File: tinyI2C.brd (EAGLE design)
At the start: 100 x 80 mm, 0 parts

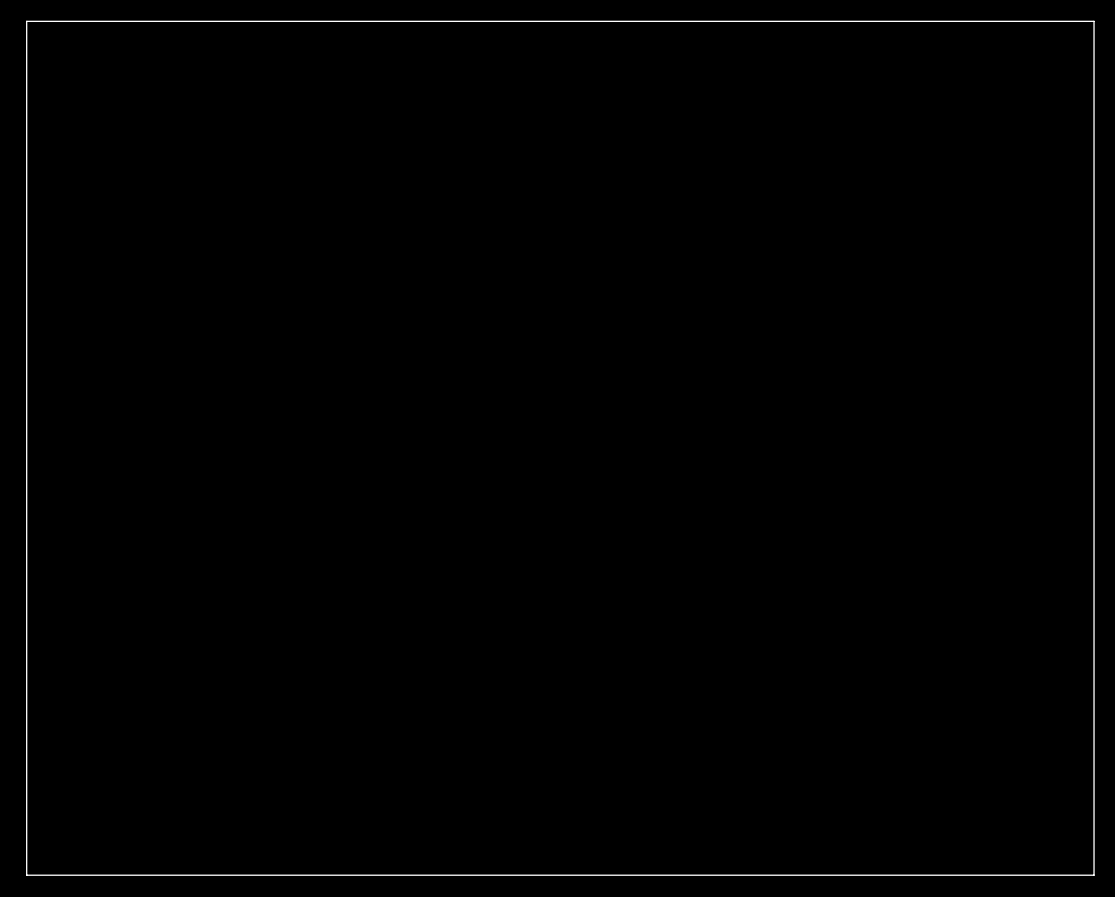
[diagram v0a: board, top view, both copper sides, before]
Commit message: sch and brd update
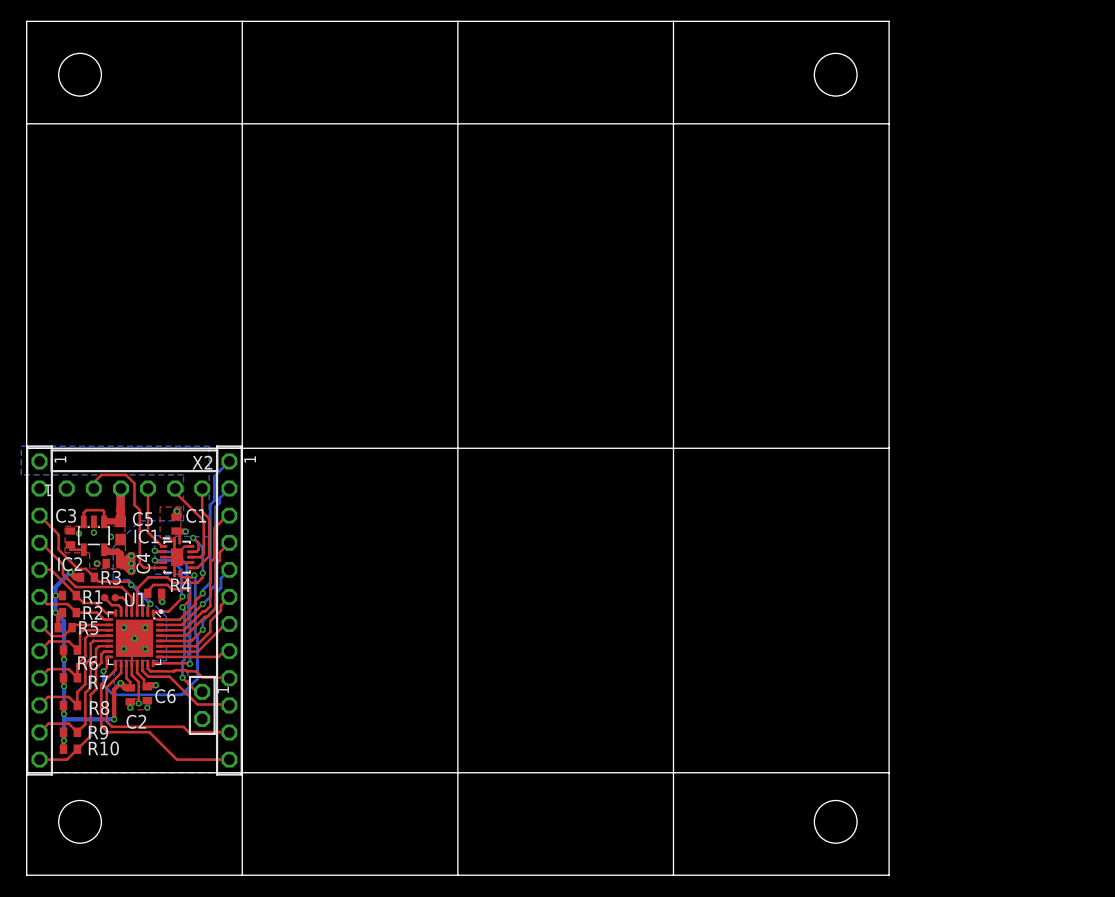
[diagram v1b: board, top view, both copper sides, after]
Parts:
- added C1, C2, C3, C4, C6: 1005, rcl:C1005
- added C5: 1608, rcl:C1608
- added IC1: 74ABT125BQ, 74xx-eu_local:DHVQFN14
- added IC2: TPS76318, texas:SOT23-DBV
- added R1, R2: 220/1005, rcl:R1005
- added R10, R3, R4, R5, R6, R7, R8, R9: 10k/1005, rcl:R1005
- added TP1, TP2, TP3, TP8, TP9: TPTP07R, testpad:TP07R
- added U1: LPC824M201JHI33, mbed-HDK:HVQFN33
- added X1, X3: TSW-112-02-S-S, con-samtec.local:TSW-112-02-S-S
- added X2: TSW-106-02-S-S-RA, con-samtec.local:TSW-106-02-S-S-RA
- added X4: TSW-102-02-S-S, con-samtec.local:TSW-102-02-S-S
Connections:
- new net !ISP!: R3.1, U1.2, X1.3
- new net !RESET!: R4.1, U1.3, X4.1
- new net 1.8V: C1.1, C2.1, C4.1, C6.1, IC1.14, IC2.5, R1.2, R10.2, R2.2, R3.2, R4.2, R5.2, R6.2, R7.2, R8.2, R9.2, TP2.TP, U1.19, U1.21, X1.1
- new net 5V: C5.1, IC2.1, IC2.3, TP1.TP, X2.3
- new net CTS<-: IC1.6, X2.2
- new net GND: C1.2, C2.2, C3.2, C4.2, C5.2, C6.2, IC1.1, IC1.10, IC1.13, IC1.4, IC1.7, IC1.EXP, IC2.2, TP3.TP, U1.20, U1.EXP, X1.2, X2.1, X4.2
- new net GPIO00: U1.32, X3.1
- new net GPIO01: U1.31, X3.2
- new net GPIO02: U1.30, X3.3
- new net GPIO03: U1.29, X3.4
- new net GPIO04: U1.28, X3.5
- new net GPIO05: U1.27, X3.6
- new net GPIO06: U1.26, X3.7
- new net GPIO07: U1.25, X3.8
- new net GPIO10: R10.1, U1.15, X1.12
- new net GPIO11: R9.1, U1.14, X1.11
- new net GPIO12: R8.1, U1.13, X1.10
- new net GPIO13: R7.1, U1.12, X1.9
- new net GPIO14: R6.1, U1.11, X1.8
- new net GPIO15: R5.1, U1.10, X1.7
- new net GPIO16: U1.5, X1.4
- new net I2C_SCL: R2.1, U1.9, X1.6
- new net I2C_SDA: R1.1, U1.8, X1.5
- new net N$1: C3.1, IC2.4
- new net RTS->: IC1.9, X2.6
- new net RX<-: IC1.11, X2.5
- new net SPI_CS: U1.17, X3.12
- new net SPI_MISO: U1.22, X3.10
- new net SPI_MOSI: U1.23, X3.9
- new net SPI_SCK: U1.18, X3.11
- new net SWCLK: TP8.TP, U1.6
- new net SWDIO: TP9.TP, U1.7
- new net TGT_CTS: IC1.8, U1.16
- new net TGT_RTS: IC1.5, U1.1
- new net TGT_RX: IC1.3, U1.24
- new net TGT_TX: IC1.12, U1.4
- new net TX->: IC1.2, X2.4
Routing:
- net 1.8V: track 0.00 -> 49.3 mm, vias 0 -> 15
- net TGT_CTS: track 0.00 -> 24.3 mm, vias 0 -> 2
- net SPI_CS: track 0.00 -> 19.7 mm
- net GPIO00: track 0.00 -> 18.6 mm, vias 0 -> 1
- net SPI_SCK: track 0.00 -> 17.9 mm
- net !RESET!: track 0.00 -> 17.8 mm, vias 0 -> 2
- net TGT_RX: track 0.00 -> 17.3 mm, vias 0 -> 2
- net GPIO01: track 0.00 -> 16.7 mm, vias 0 -> 1
- net !ISP!: track 0.00 -> 15.6 mm, vias 0 -> 2
- net GND: track 0.00 -> 15.6 mm, vias 0 -> 13
- net TGT_TX: track 0.00 -> 15.5 mm, vias 0 -> 2
- net CTS<-: track 0.00 -> 15.1 mm
- net GPIO02: track 0.00 -> 15.0 mm
- net GPIO10: track 0.00 -> 14.6 mm
- net GPIO11: track 0.00 -> 14.1 mm
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- added copper zone on layer 16, net 1.8V
- added copper zone on layer 1, net GND
- added copper zone on layer 16, net GND
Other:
- board size 100 x 80 mm -> 80.8 x 80 mm
